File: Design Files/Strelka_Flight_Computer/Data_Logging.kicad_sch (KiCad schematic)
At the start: 7 parts, among them IC1 XTSD04GLGEAG

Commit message: Creating BOM
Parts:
- IC1: Height 0.95 -> (none); LCSC# (none) -> C558839; Manufacturer_Name XTX -> (none); Manufacturer_Part_Number XTSD04GLGEAG -> (none)
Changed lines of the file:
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@@
       (effects (font (size 1.27 1.27)) (justify left) hide)
     )
-    (property "Description" "LGA8-8x6mm FLASH" (id 4) (at 104.775 53.34 0)
-      (effects (font (size 1.27 1.27)) (justify left) hide)
-    )
-    (property "Height" "0.95" (id 5) (at 104.775 55.88 0)
-      (effects (font (size 1.27 1.27)) (justify left) hide)
-    )
-    (property "Manufacturer_Name" "XTX" (id 6) (at 104.775 58.42 0)
-      (effects (font (size 1.27 1.27)) (justify left) hide)
-    )
-    (property "Manufacturer_Part_Number" "XTSD04GLGEAG" (id 7) (at 104.775 60.96 0)
-      (effects (font (size 1.27 1.27)) (justify left) hide)
-    )
-    (property "Mouser Part Number" "" (id 8) (at 104.775 63.5 0)
-      (effects (font (size 1.27 1.27)) (justify left) hide)
-    )
-    (property "Mouser Price/Stock" "" (id 9) (at 104.775 66.04 0)
-      (effects (font (size 1.27 1.27)) (justify left) hide)
-    )
-    (property "Arrow Part Number" "" (id 10) (at 104.775 68.58 0)
-      (effects (font (size 1.27 1.27)) (justify left) hide)
-    )
-    (property "Arrow Price/Stock" "" (id 11) (at 104.775 71.12 0)
-      (effects (font (size 1.27 1.27)) (justify left) hide)
+    (property "LCSC#" "C558839" (id 4) (at 45.085 50.8 0)
+      (effects (font (size 1.27 1.27)) hide)
     )
     (pin "1")

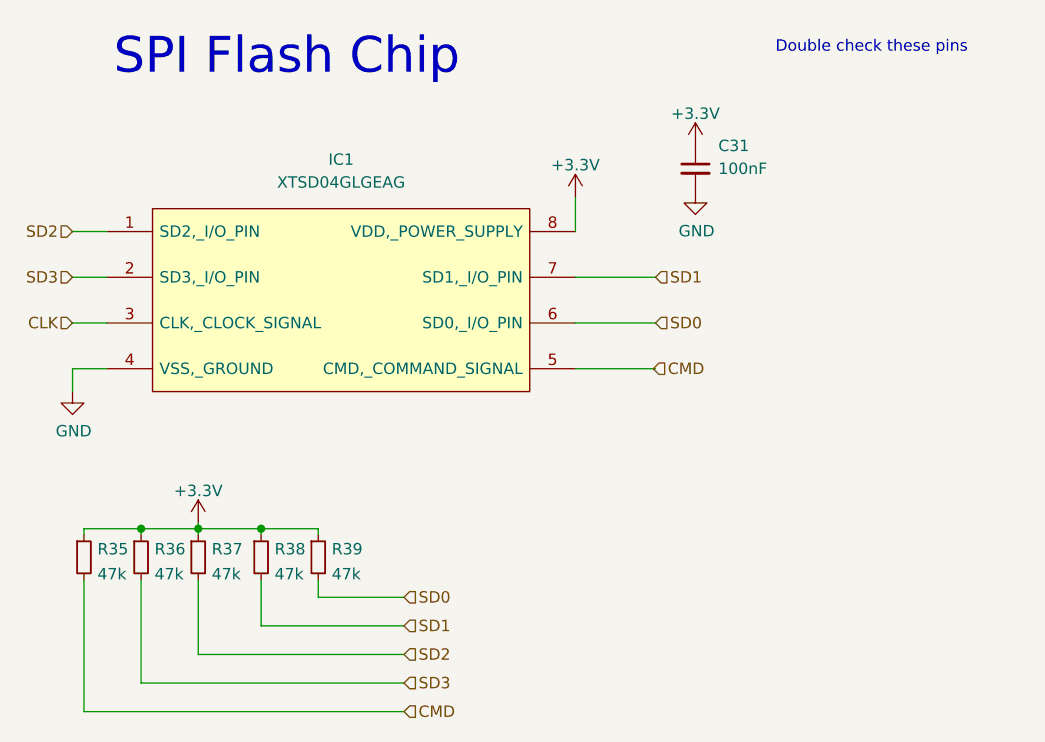
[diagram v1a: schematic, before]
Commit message: redo placement
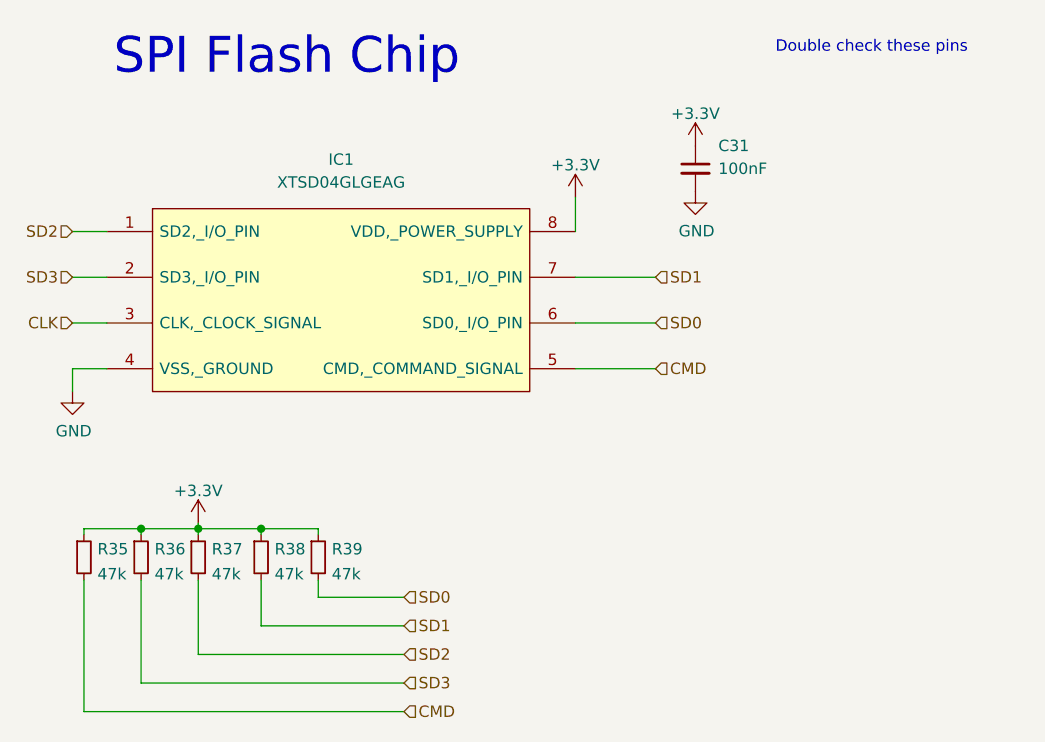
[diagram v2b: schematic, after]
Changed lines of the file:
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@@
     (effects (font (size 1.27 1.27)) (justify right))
   )
-  (hierarchical_label "CMD" (shape input) (at 105.8054 58.42 0)
+  (hierarchical_label "CMD" (shape input) (at 106.045 58.42 0)
     (effects (font (size 1.27 1.27)) (justify left))
   )
